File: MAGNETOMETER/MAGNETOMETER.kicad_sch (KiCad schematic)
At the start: 3 parts, among them IC6 MMC5603NJ, J1 M80-8770405

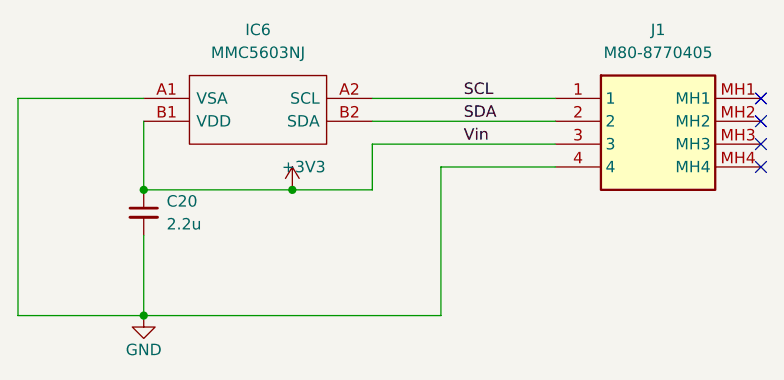
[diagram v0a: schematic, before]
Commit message: Done with most of the boards
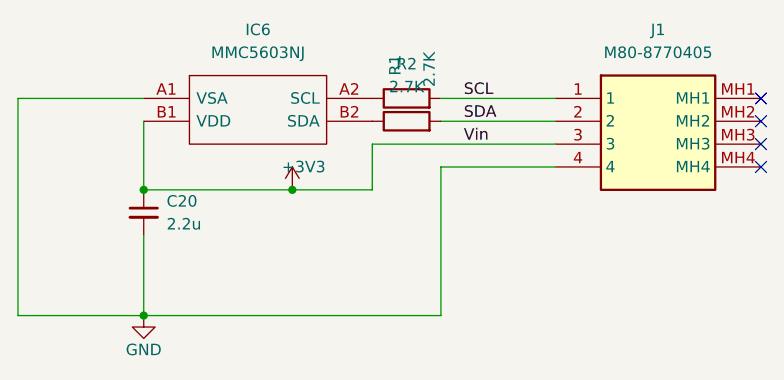
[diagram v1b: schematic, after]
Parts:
- added R1, R2: 2.7K, Resistor_SMD:R_0201_0603Metric, symbol Device:R
- J1: footprint M808770405 -> KiCad:M808770405
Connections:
- net SCL: now also R1.2; no longer IC6.A2 (SCL)
- net SDA: now also R2.2; no longer IC6.B2 (SDA)
- new net: IC6.A2 (SCL), R1.1
- new net: IC6.B2 (SDA), R2.1
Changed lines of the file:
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@@
   (no_connect (at 186.69 90.17))
   (no_connect (at 186.69 85.09))
-  (wire (pts (xy 143.51 87.63) (xy 163.83 87.63))
-    (stroke (width 0) (type default))
-  )
   (wire (pts (xy 151.13 109.22) (xy 151.13 92.71))
     (stroke (width 0) (type default))
@@
     (stroke (width 0) (type default))
   )
-  (wire (pts (xy 143.51 85.09) (xy 163.83 85.09))
+  (wire (pts (xy 151.13 87.63) (xy 163.83 87.63))
     (stroke (width 0) (type default))
   )
   (wire (pts (xy 151.13 92.71) (xy 163.83 92.71))
+    (stroke (width 0) (type default))
+  )
+  (wire (pts (xy 151.13 85.09) (xy 163.83 85.09))
     (stroke (width 0) (type default))
   )
@@
         (path "/39d7ebb3-b69d-4ae9-8f55-c9acfe77d345/82e19a29-2001-4834-a54c-a35440bfa66f"
           (reference "C20") (unit 1)
+        )
+      )
+    )
+  )
+  (symbol (lib_id "Device:R") (at 147.32 85.09 90) (unit 1)
+    (in_bom yes) (on_board yes) (dnp no)
+    (property "Reference" "R1" (at 146.05 82.55 0)
+      (effects (font (size 1.27 1.27)) (justify left))
+    )
+    (property "Value" "2.7K" (at 149.86 83.82 0)
+      (effects (font (size 1.27 1.27)) (justify left))
+    )
+    (property "Footprint" "Resistor_SMD:R_0201_0603Metric" (at 147.32 86.868 90)
+      (effects (font (size 1.27 1.27)) hide)
+    )
+    (property "Datasheet" "~" (at 147.32 85.09 0)
+      (effects (font (size 1.27 1.27)) hide)
+    )
+    (pin "1")
+    (pin "2")
+    (instances
+      (project "MAGNETOMETER"
+        (path "/1ff82954-21a9-4f7a-99bd-a8202cea8bb4"
+          (reference "R1") (unit 1)
         )
       )
@@
         (path "/6135eb53-87c0-4516-a6dc-aa2a3e58fdeb"
           (reference "#PWR02") (unit 1)
+        )
+      )
+    )
+  )
+  (symbol (lib_id "Device:R") (at 147.32 87.63 90) (unit 1)
+    (in_bom yes) (on_board yes) (dnp no) (fields_autoplaced)
+    (property "Reference" "R2" (at 147.32 81.28 90)
+      (effects (font (size 1.27 1.27)))
+    )
+    (property "Value" "2.7K" (at 147.32 83.82 90)
+      (effects (font (size 1.27 1.27)))
+    )
+    (property "Footprint" "Resistor_SMD:R_0201_0603Metric" (at 147.32 89.408 90)
+      (effects (font (size 1.27 1.27)) hide)
+    )
+    (property "Datasheet" "~" (at 147.32 87.63 0)
+      (effects (font (size 1.27 1.27)) hide)
+    )
+    (pin "1")
+    (pin "2")
+    (instances
+      (project "MAGNETOMETER"
+        (path "/1ff82954-21a9-4f7a-99bd-a8202cea8bb4"
+          (reference "R2") (unit 1)
         )
       )
@@
       (effects (font (size 1.27 1.27)))
     )
-    (property "Footprint" "M808770405" (at 182.88 180.01 0)
+    (property "Footprint" "KiCad:M808770405" (at 182.88 180.01 0)
       (effects (font (size 1.27 1.27)) (justify left top) hide)
     )
